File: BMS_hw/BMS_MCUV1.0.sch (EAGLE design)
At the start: 1 part

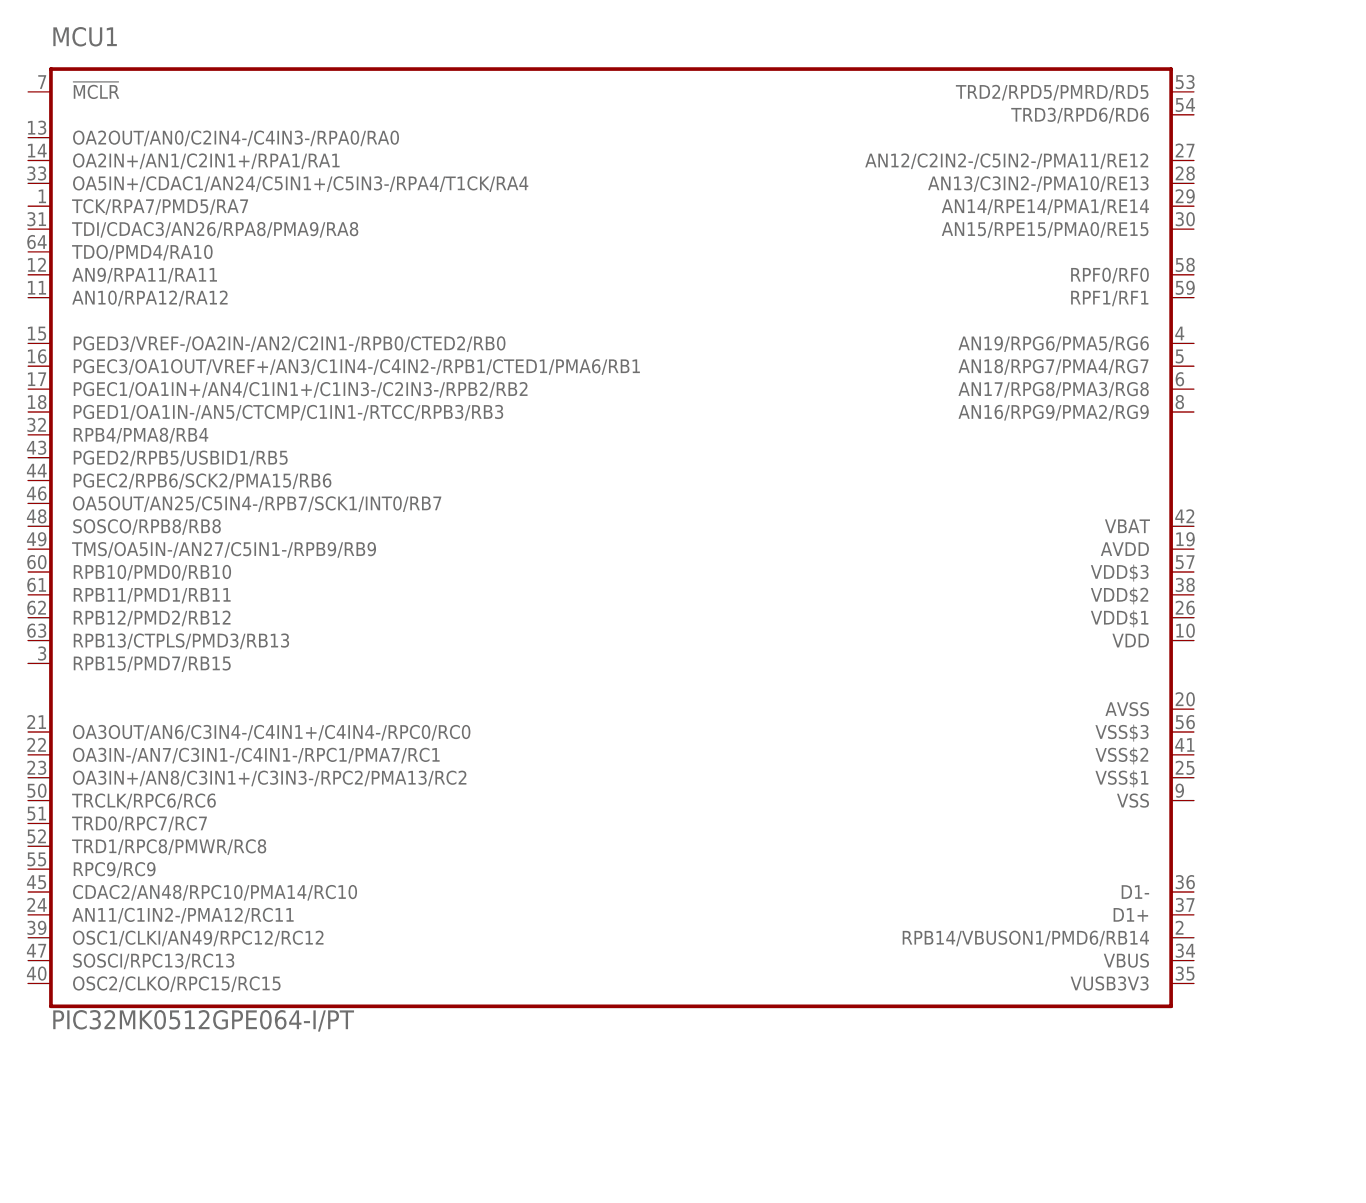
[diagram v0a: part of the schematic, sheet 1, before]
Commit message: Revert "Merge branch 'hw' of https://github.com/kunal-GF/GF_BMS into hw"
This reverts commit cb819c5a256ea6b478828d222d8978a164d41654, reversing
changes made to 1a0582993ac0a8851db6f9d974378484a723c9b0.
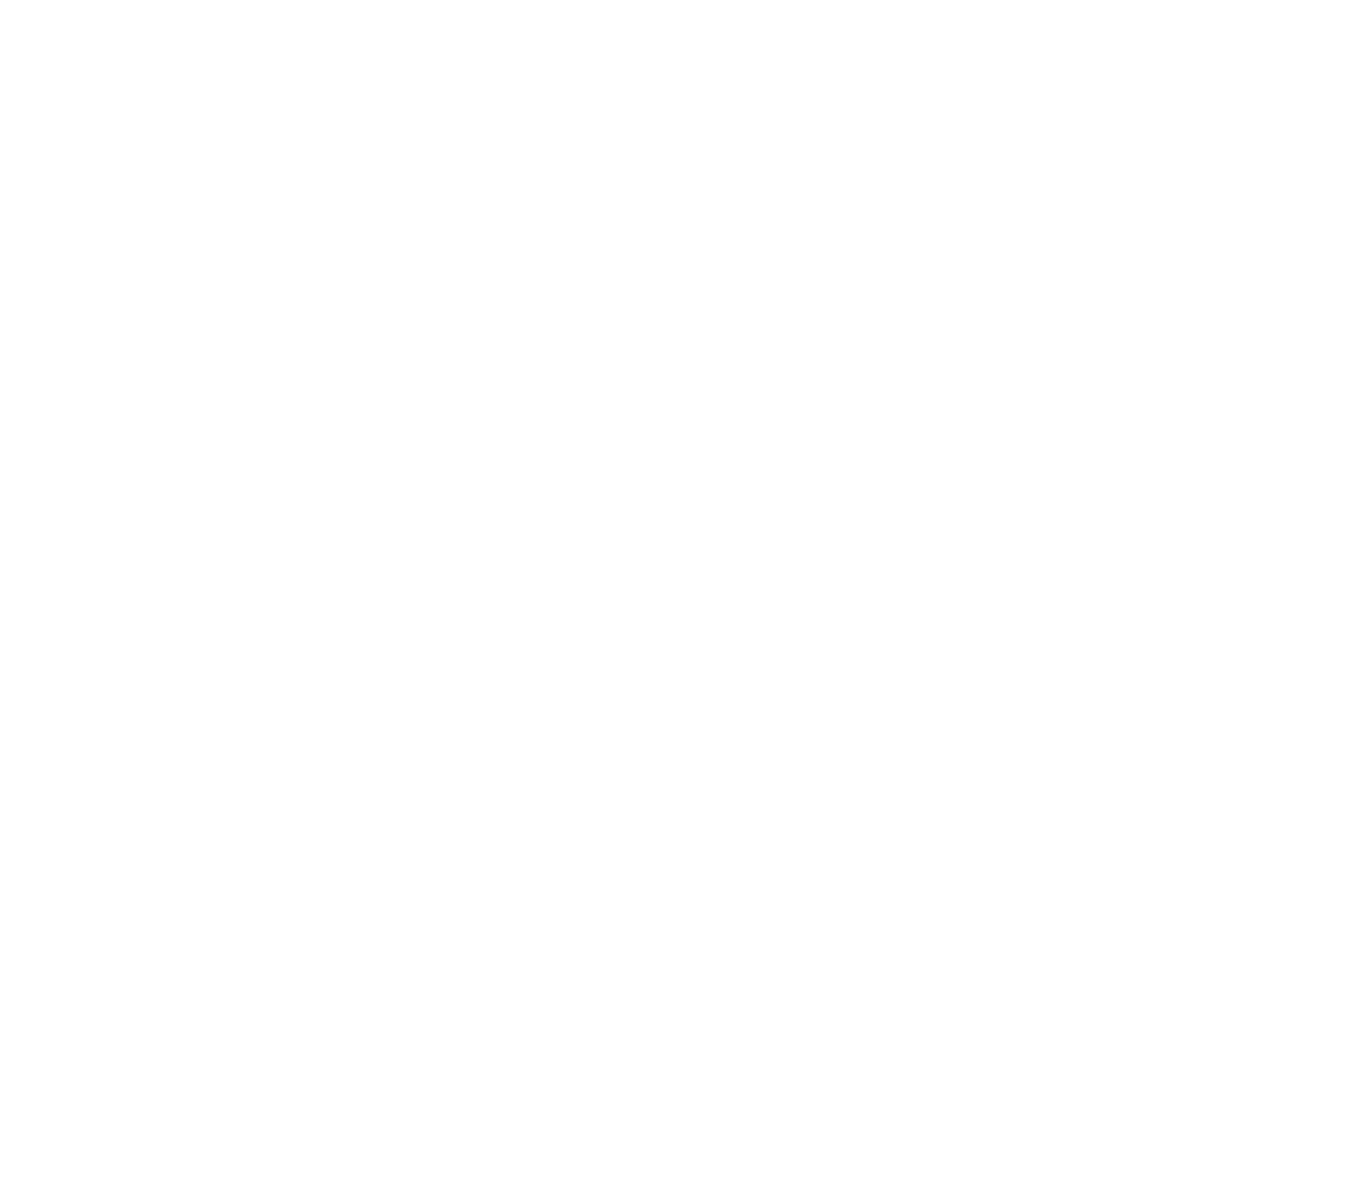
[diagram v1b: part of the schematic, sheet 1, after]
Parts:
- removed MCU1: PIC32MK0512GPE064-I/PT, GreenFuel:PIC32MK0512GPE064-I/PT
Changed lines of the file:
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@@
 <setting verticaltext="up"/>
 </settings>
-<grid distance="0.1" unitdist="inch" unit="inch" style="lines" multiple="1" display="yes" altdistance="0.01" altunitdist="inch" altunit="inch"/>
+<grid distance="0.1" unitdist="inch" unit="inch" style="lines" multiple="1" display="no" altdistance="0.01" altunitdist="inch" altunit="inch"/>
 <layers>
 <layer number="1" name="Top" color="4" fill="1" visible="no" active="no"/>
@@
 <part name="FRAME1" library="frames" library_urn="urn:adsk.eagle:library:229" deviceset="A3L-LOC" device=""/>
 <part name="FRAME2" library="frames" library_urn="urn:adsk.eagle:library:229" deviceset="A3L-LOC" device=""/>
-<part name="MCU1" library="GreenFuel" deviceset="PIC32MK0512GPE064-I/PT" device=""/>
 </parts>
 <sheets>
@@
 <instances>
 <instance part="FRAME1" gate="G$1" x="0" y="0"/>
-<instance part="MCU1" gate="G$1" x="190.5" y="142.24"/>
 </instances>
 <busses>
